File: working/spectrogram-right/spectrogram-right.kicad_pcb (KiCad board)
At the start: 2 copper layers, 159.5 x 99.4 mm, 154 parts, among them P1 TC2030-IDC, U1 TRRS, U2 ProMicro

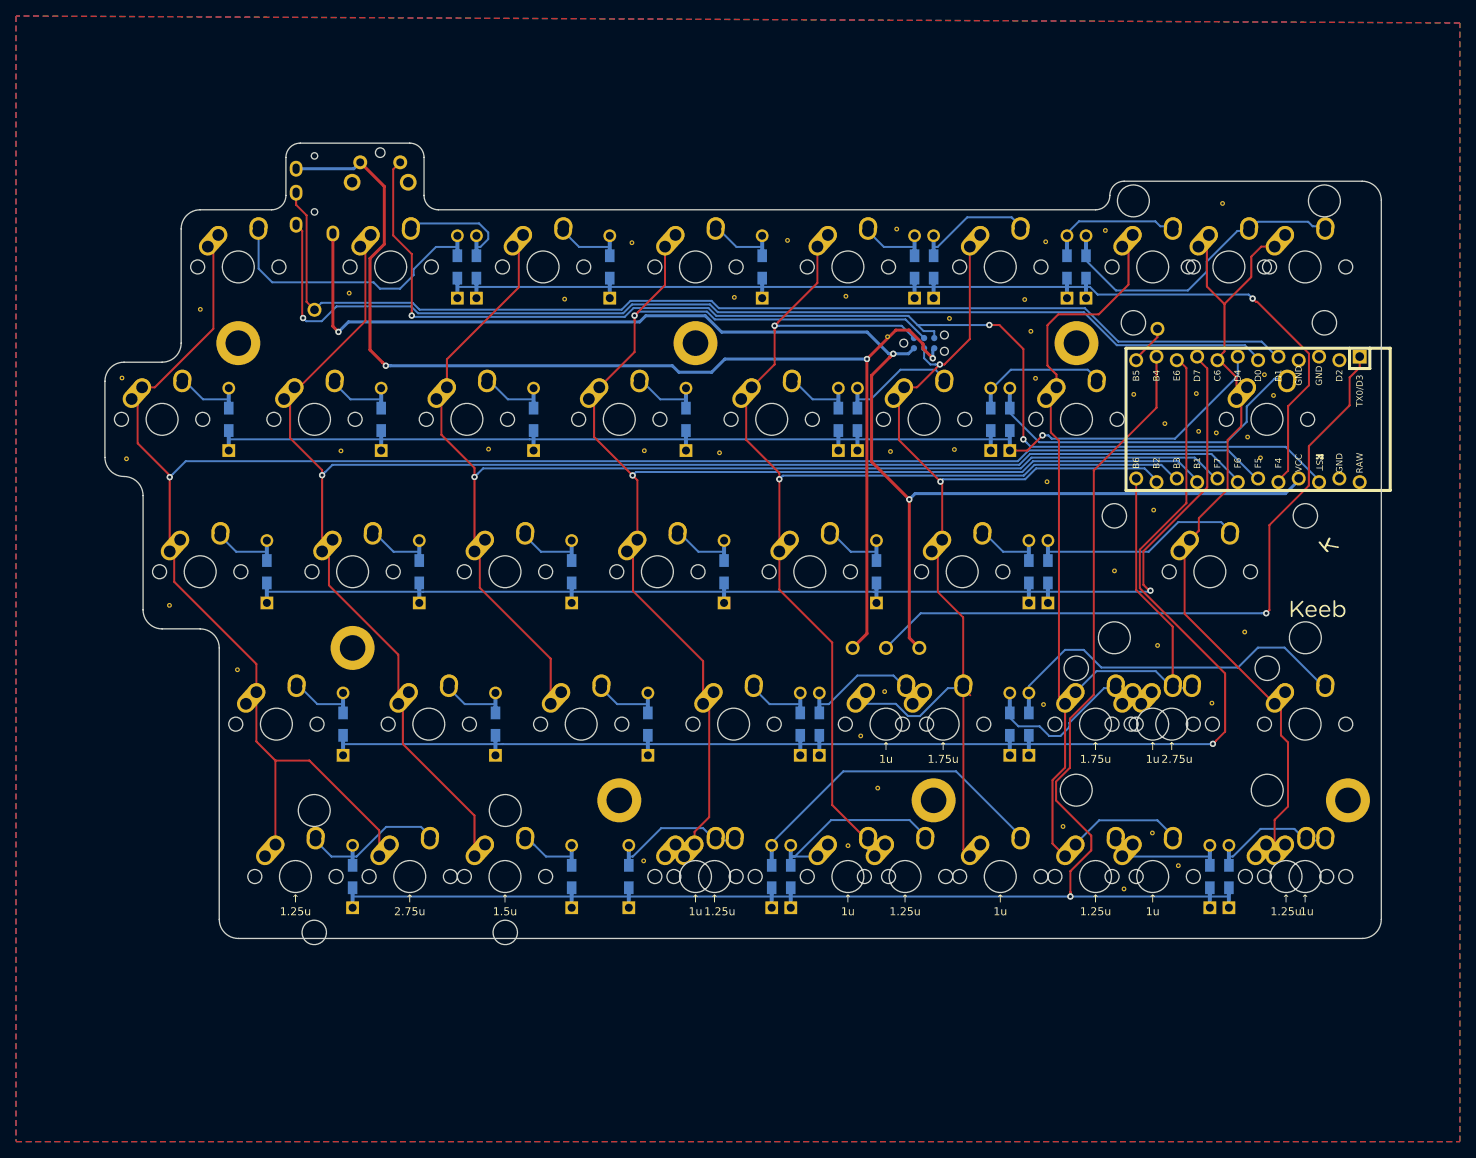
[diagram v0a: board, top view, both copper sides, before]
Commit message: Pushed updtes
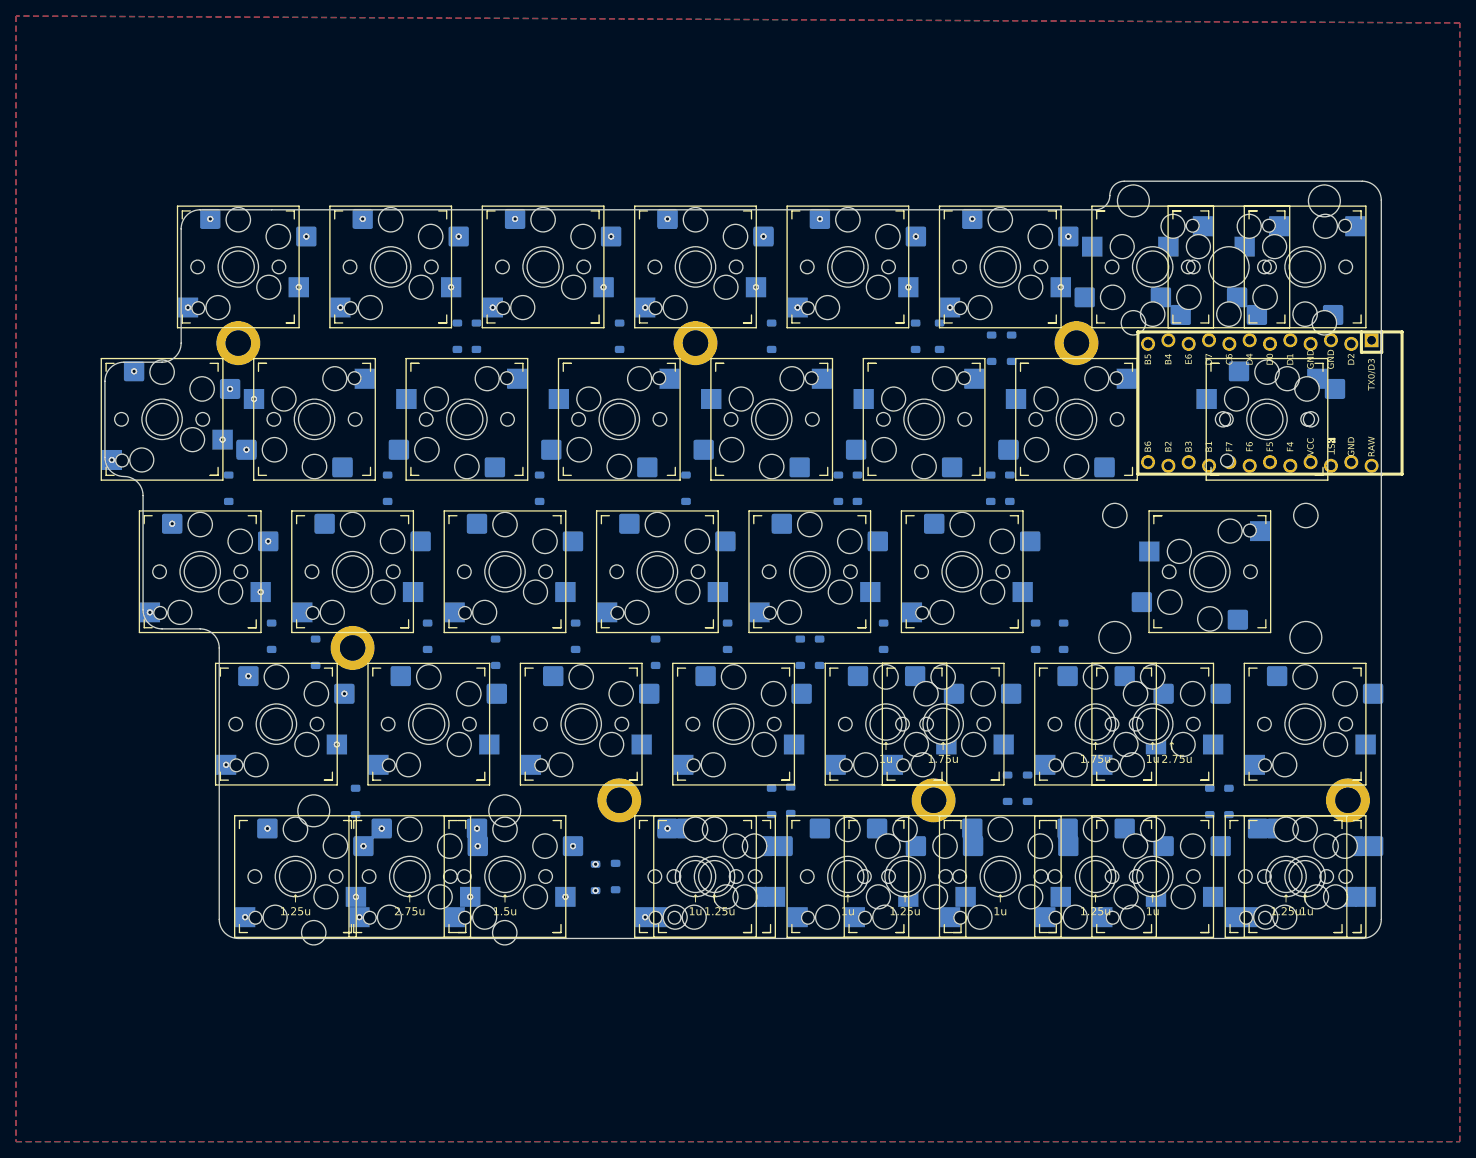
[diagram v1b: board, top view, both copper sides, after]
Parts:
- removed G*** (x2): LOGO, Keebio-Art:AIRI-Logo2
- removed G*** (x2): LOGO, Keebio-Art:Keebio-TwoTone
- removed P1: TC2030-IDC, Tag-Connect:TC2030-NL_SMALL
- removed REF** (x51): VIA-0.6mm, Keebio-Parts:VIA-0.6mm
- removed SW_D7: SW_Push, MX_Alps_Hybrid:MX-2.75U-NoLED
- removed SW_R1: Reset, Keebio-Parts:SW_Tactile_SPST_Angled_MJTP1117
- removed TP1: VCC, Keebio-Parts:SinglePad
- removed TP3: GND, Keebio-Parts:SinglePad
- removed TP4: RGB, Keebio-Parts:SinglePad
- removed TP5: B5, Keebio-Parts:SinglePad
- removed TP6: Extra Data, Keebio-Parts:SinglePad
- removed U1: TRRS, Keebio-Parts:TRRS-PJ-320A
- D_A1, D_A2, D_A3, D_A4, D_A5, D_A6, D_A7, D_A8, D_B1, D_B2, D_B3, D_B4, D_B5, D_B6, D_B7, D_B8, D_C1, D_C2, D_C3, D_C4, D_C5, D_C6, D_C8, D_D1, D_D2, D_D3, D_D4, D_D6, D_D7, D_D8, D_E1, D_E2, D_E4, D_E5, D_E6, D_E7, D_E8: footprint Keebio-Parts:Diode-Hybrid-Back -> Diode_SMD:D_SOD-123; moved to B.Cu
- SW_A1, SW_A2, SW_A3, SW_A4, SW_A5, SW_A6, SW_A7, SW_AB8, SW_B1, SW_B2, SW_B3, SW_B4, SW_B5, SW_B6, SW_B7, SW_C1, SW_C2, SW_C3, SW_C4, SW_C5, SW_C6, SW_D1, SW_D2, SW_D3, SW_D4, SW_D6, SW_DB8, SW_DC7, SW_EB4, SW_EB5, SW_EB6, SW_EB7, SW_EB8: footprint MX_Alps_Hybrid:MX-1U-NoLED -> jakestuff:ChocMX_flippedpads
- SW_A8: footprint MX_Alps_Hybrid:MX-2U-ReversedStabilizers-NoLED -> jakestuff:ChocMX_flippedpads_2.25U
- SW_B8: footprint MX_Alps_Hybrid:MX-1.5U-NoLED -> jakestuff:ChocMX_sameside_flippedpads
- SW_C8: footprint MX_Alps_Hybrid:MX-2.25U-NoLED -> jakestuff:ChocMX_flippedpads_2.25U_reversedstab
- SW_DB7, SW_DC6: footprint MX_Alps_Hybrid:MX-1.75U-NoLED -> jakestuff:ChocMX_flippedpads
- SW_E1: footprint MX_Alps_Hybrid:MX-2.75U-ReversedStabilizers-NoLED -> jakestuff:ChocMX_flippedpads_2.25U_reversedstab
- SW_E2: footprint MX_Alps_Hybrid:MX-1.5U-NoLED -> jakestuff:ChocMX_flippedpads
- SW_E4, SW_E5, SW_E7, SW_E8, SW_EB1: footprint MX_Alps_Hybrid:MX-1.25U-NoLED -> jakestuff:ChocMX_flippedpads
- moved D_A7 13.9 mm to (127.5, 43.5)
- moved D_A8 13.8 mm to (130.0, 43.5)
- moved D_D1 9.62 mm to (43.0, 81.5)
- moved D_E5 9.54 mm to (102.4, 100.0)
- moved D_E1 9.39 mm to (48.0, 100.2)
- moved D_E6 9.39 mm to (100.0, 100.2)
- moved D_E8 9.39 mm to (157.2, 100.2)
- moved D_E7 9.39 mm to (154.8, 100.2)
- moved D_D3 9.04 mm to (85.5, 81.5)
- moved D_D6 8.99 mm to (106.0, 81.5)
- moved D_D2 8.99 mm to (65.5, 81.5)
- moved D_D4 8.99 mm to (103.6, 81.5)
- moved D_A3 8.75 mm to (81.0, 42.0)
- moved D_A4 8.74 mm to (100.0, 42.0)
- moved D_A6 8.69 mm to (121.0, 42.0)
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- renumbered H6 to H7
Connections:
- U2 pad 24: (no net) -> unconnected-(U2-RAW-Pad24)
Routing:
- net Col1: track 246.4 -> 0.00 mm, vias 1 -> 12
- net Col2: track 207.7 -> 0.00 mm, vias 1 -> 6
- net Col4: track 197.1 -> 0.00 mm
- net RowE: track 185.6 -> 0.00 mm
- net VCC: track 177.7 -> 0.00 mm, vias 3 -> 0
- net RowD: track 164.9 -> 0.00 mm, vias 1 -> 0
- net Col3: track 160.7 -> 0.00 mm, vias 1 -> 2
- net Col5: track 154.1 -> 0.00 mm
- net Reset: track 153.2 -> 0.00 mm, vias 3 -> 0
- net GND: track 147.5 -> 0.00 mm, vias 3 -> 0
- net Col7: track 145.6 -> 0.00 mm
- net RowC: track 143.8 -> 0.00 mm, vias 1 -> 0
- net Data2: track 140.2 -> 0.00 mm
- net Data: track 135.9 -> 0.00 mm, vias 1 -> 0
- net Col6: track 133.0 -> 0.00 mm
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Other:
- board size 159.5 x 99.4 mm -> 159.5 x 94.7 mm
- net class Default removed
- net class Power Tracks removed
- board text added: "${REFERENCE}"
- board text added: "${VALUE}"
